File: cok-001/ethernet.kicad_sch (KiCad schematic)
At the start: 1 part, among them J3501 RJ45_Amphenol_RJMG1BD3B8K1ANR

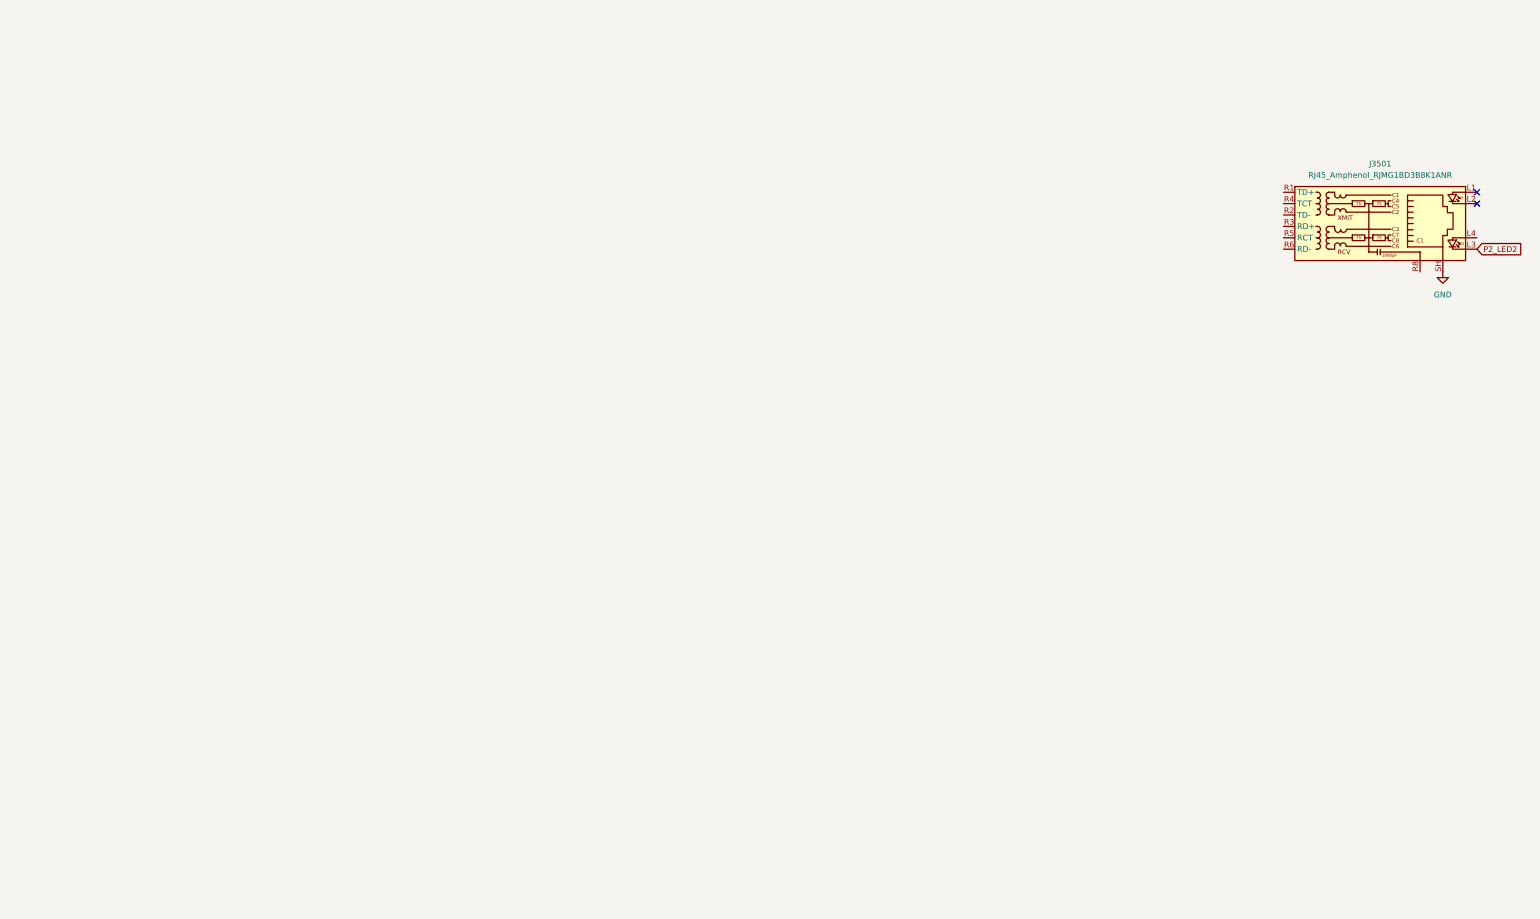
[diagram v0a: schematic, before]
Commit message: ethernet
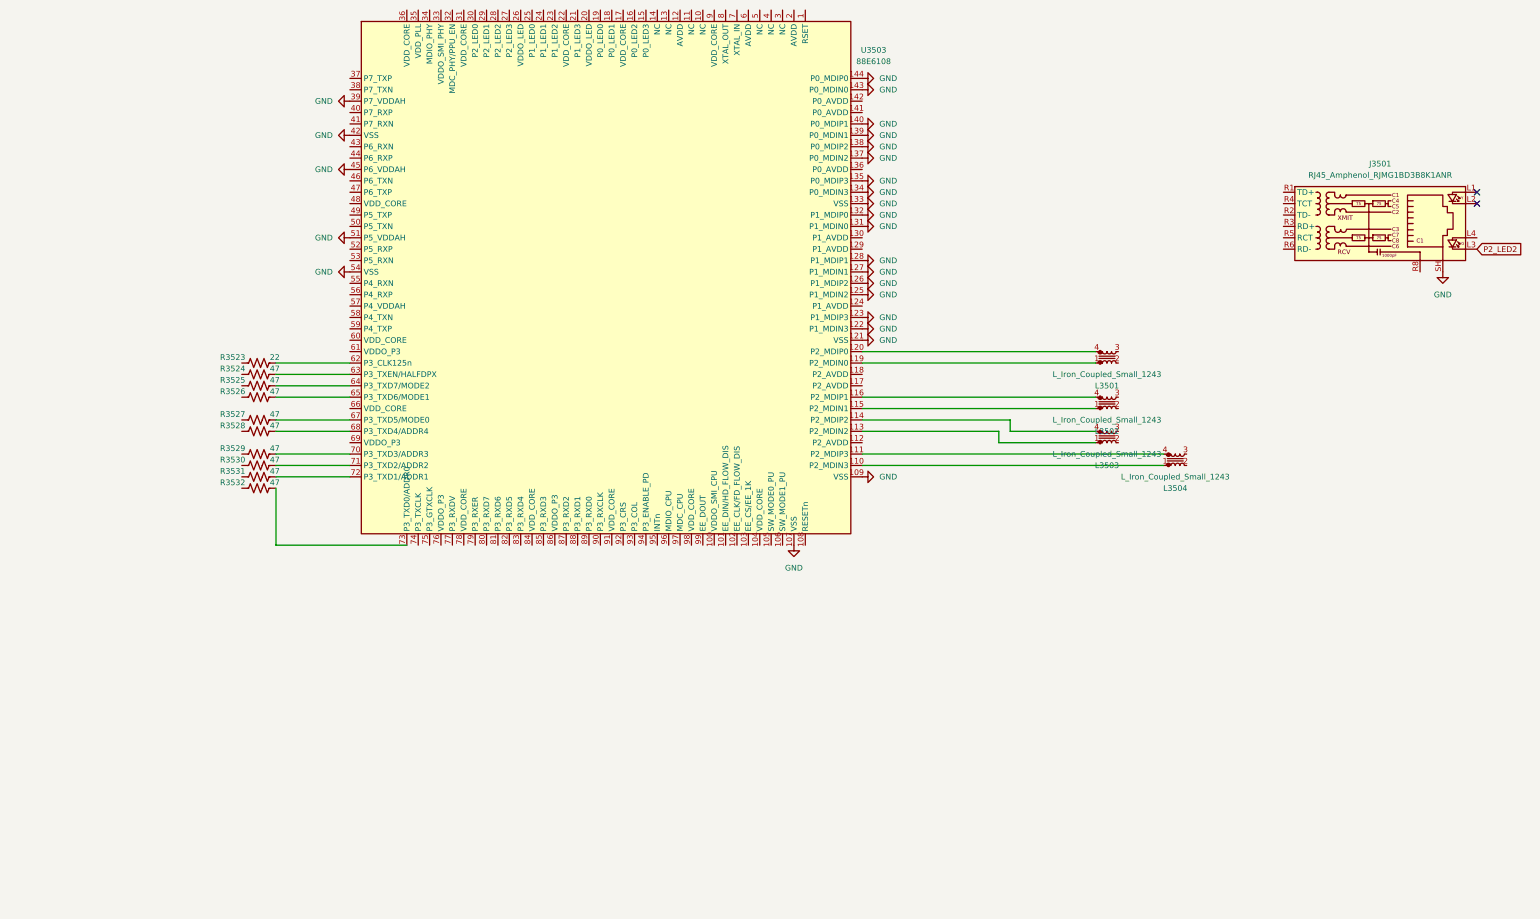
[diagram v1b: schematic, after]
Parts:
- added L3501, L3502, L3503, L3504: L_Iron_Coupled_Small_1243, Inductor_SMD:L_CommonModeChoke_Coilcraft_0805USB, symbol Device:L_Iron_Coupled_Small_1243
- added R3523: 22, Resistor_SMD:R_0402_1005Metric, symbol Device:R_US
- added R3524, R3525, R3526, R3527, R3528, R3529, R3530, R3531, R3532: 47, Resistor_SMD:R_0402_1005Metric, symbol Device:R_US
- added U3503: 88E6108, Package_QFP:LQFP-144_20x20mm_P0.5mm, symbol PS3:88E6108
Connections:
- net GND: now also U3503.107 (VSS), U3503.109 (VSS), U3503.121 (VSS), U3503.122 (P1_MDIN3), U3503.123 (P1_MDIP3), U3503.125 (P1_MDIN2), U3503.126 (P1_MDIP2), U3503.127 (P1_MDIN1), U3503.128 (P1_MDIP1), U3503.131 (P1_MDIN0), U3503.132 (P1_MDIP0), U3503.133 (VSS), U3503.134 (P0_MDIN3), U3503.135 (P0_MDIP3), U3503.137 (P0_MDIN2), U3503.138 (P0_MDIP2), U3503.139 (P0_MDIN1), U3503.140 (P0_MDIP1), U3503.143 (P0_MDIN0), U3503.144 (P0_MDIP0), U3503.39 (P7_VDDAH), U3503.42 (VSS), U3503.45 (P6_VDDAH), U3503.51 (P5_VDDAH), U3503.54 (VSS)
- new net: R3526.2, U3503.65 (P3_TXD6/MODE1)
- new net: R3524.2, U3503.63 (P3_TXEN/HALFDPX)
- new net: L3502.1, U3503.115 (P2_MDIN1)
- new net: L3502.4, U3503.116 (P2_MDIP1)
- new net: R3525.2, U3503.64 (P3_TXD7/MODE2)
- new net: L3501.1, U3503.119 (P2_MDIN0)
- new net: L3501.4, U3503.120 (P2_MDIP0)
- new net: L3503.1, U3503.113 (P2_MDIN2)
- new net: L3503.4, U3503.114 (P2_MDIP2)
- new net: R3523.2, U3503.62 (P3_CLK125n)
- new net: R3527.2, U3503.67 (P3_TXD5/MODE0)
- new net: R3529.2, U3503.70 (P3_TXD3/ADDR3)
- new net: L3504.1, U3503.110 (P2_MDIN3)
- new net: L3504.4, U3503.111 (P2_MDIP3)
- new net: R3530.2, U3503.71 (P3_TXD2/ADDR2)
- new net: R3528.2, U3503.68 (P3_TXD4/ADDR4)
- new net: R3532.2, U3503.73 (P3_TXD0/ADDR0)
- new net: R3531.2, U3503.72 (P3_TXD1/ADDR1)

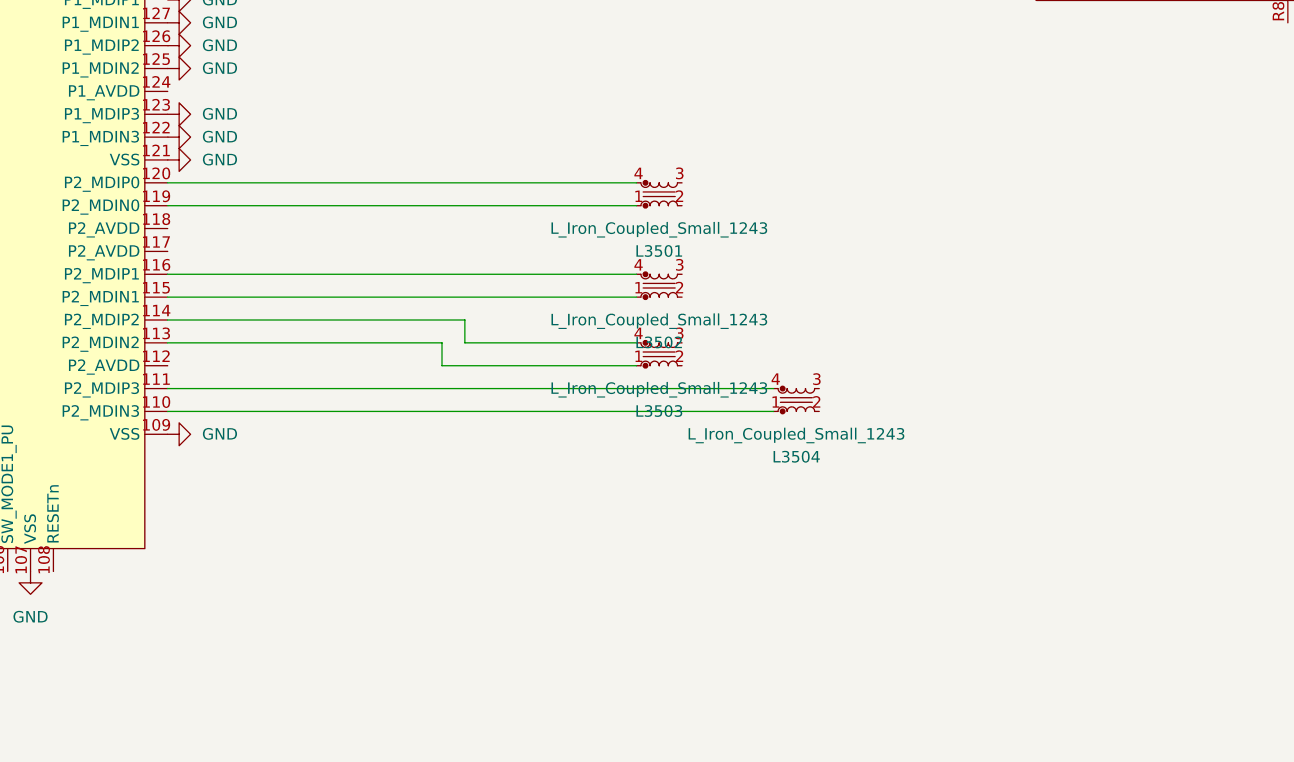
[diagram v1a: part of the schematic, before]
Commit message: av
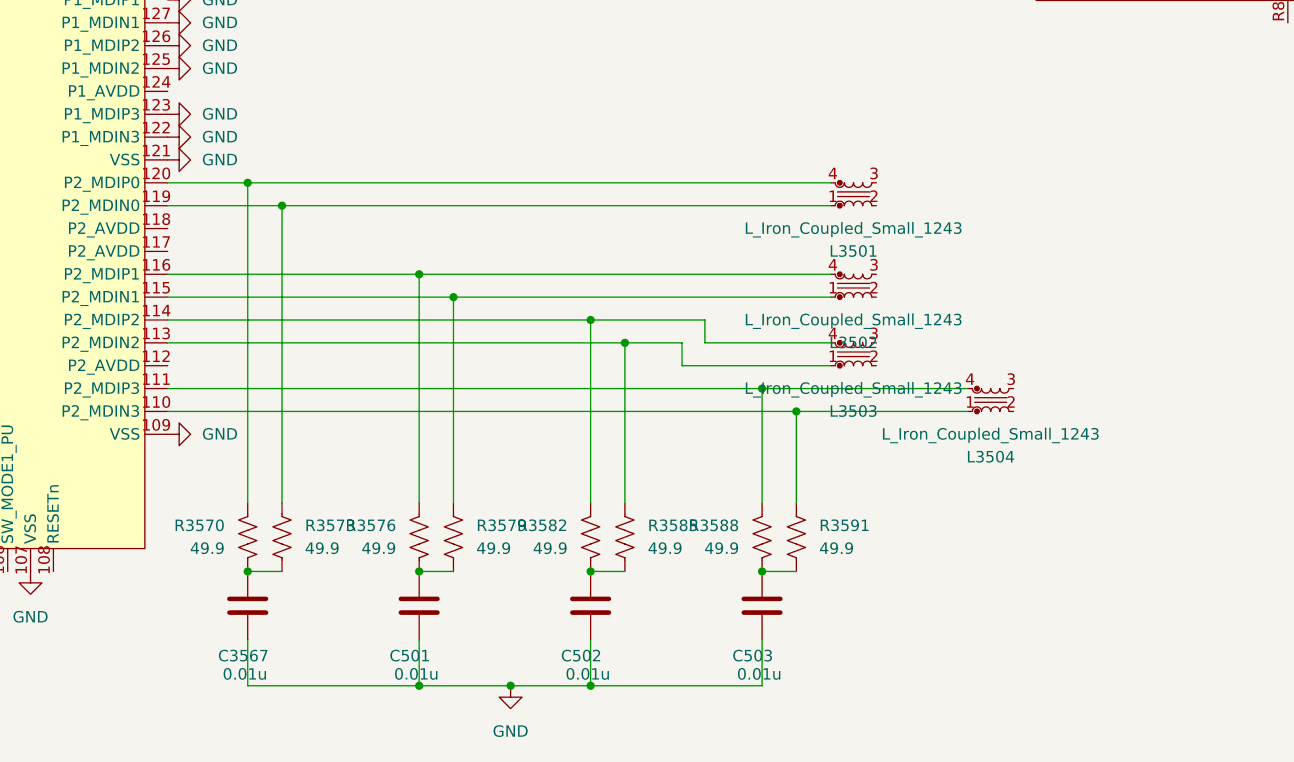
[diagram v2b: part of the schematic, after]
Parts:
- added C3567, C501, C502, C503: 0.01u, Capacitor_SMD:C_0402_1005Metric, symbol Device:C
- added R3570, R3573, R3576, R3579, R3582, R3585, R3588, R3591: 49.9, Resistor_SMD:R_0402_1005Metric, symbol Device:R_US
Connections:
- net GND: now also C3567.2, C501.2, C502.2, C503.2
- net at L3502.1, U3503.115 (P2_MDIN1): now also R3579.2
- net at L3502.4, U3503.116 (P2_MDIP1): now also R3576.2
- net at L3501.1, U3503.119 (P2_MDIN0): now also R3573.2
- net at L3501.4, U3503.120 (P2_MDIP0): now also R3570.2
- net at L3503.1, U3503.113 (P2_MDIN2): now also R3585.2
- net at L3503.4, U3503.114 (P2_MDIP2): now also R3582.2
- net at L3504.1, U3503.110 (P2_MDIN3): now also R3591.2
- net at L3504.4, U3503.111 (P2_MDIP3): now also R3588.2
- new net: C502.1, R3582.1, R3585.1
- new net: C3567.1, R3570.1, R3573.1
- new net: C503.1, R3588.1, R3591.1
- new net: C501.1, R3576.1, R3579.1
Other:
- moved on the sheet: L3501, L3502, L3503, L3504

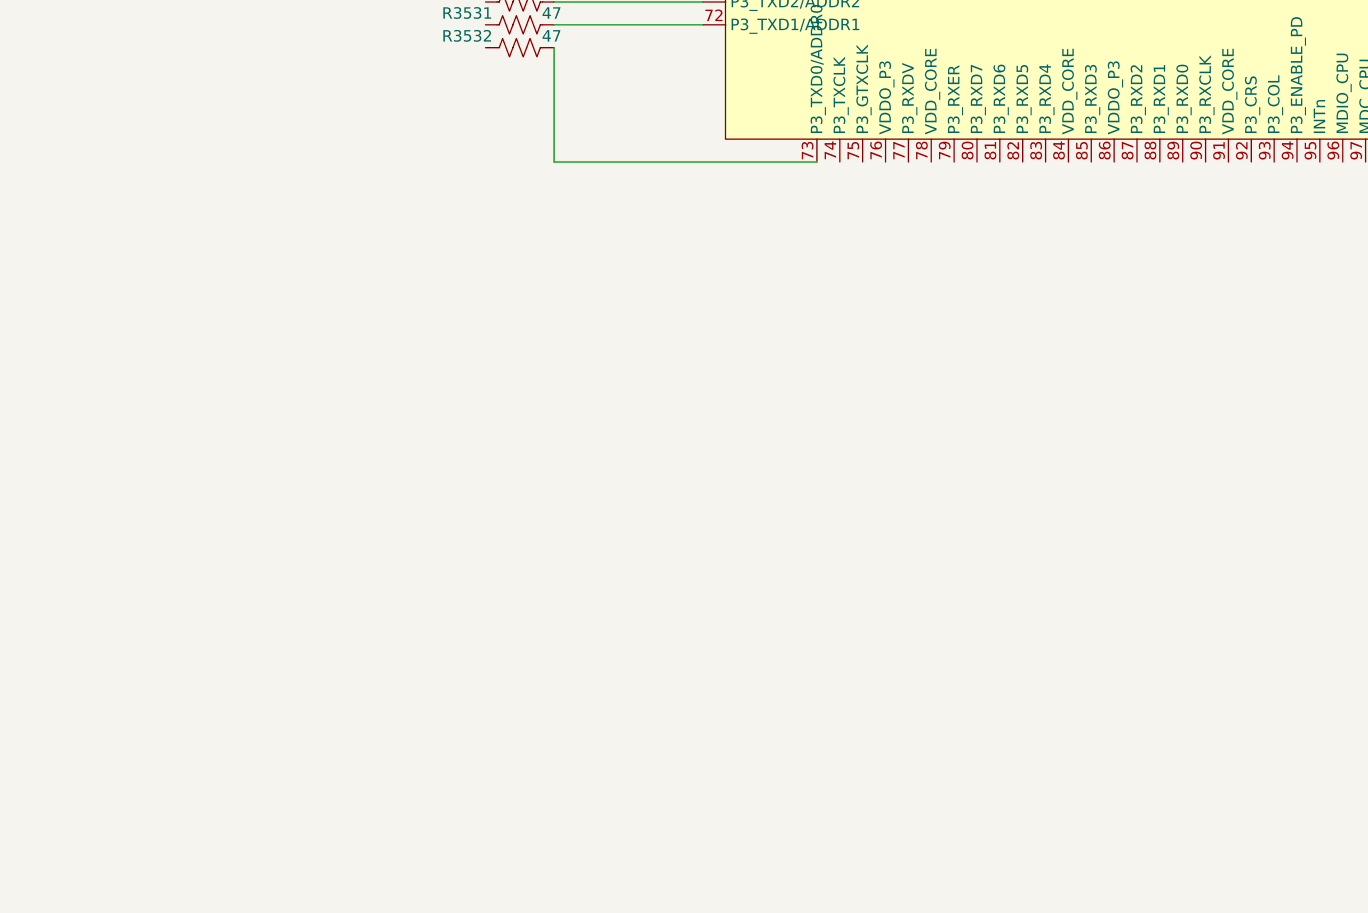
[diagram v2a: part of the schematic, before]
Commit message: aj
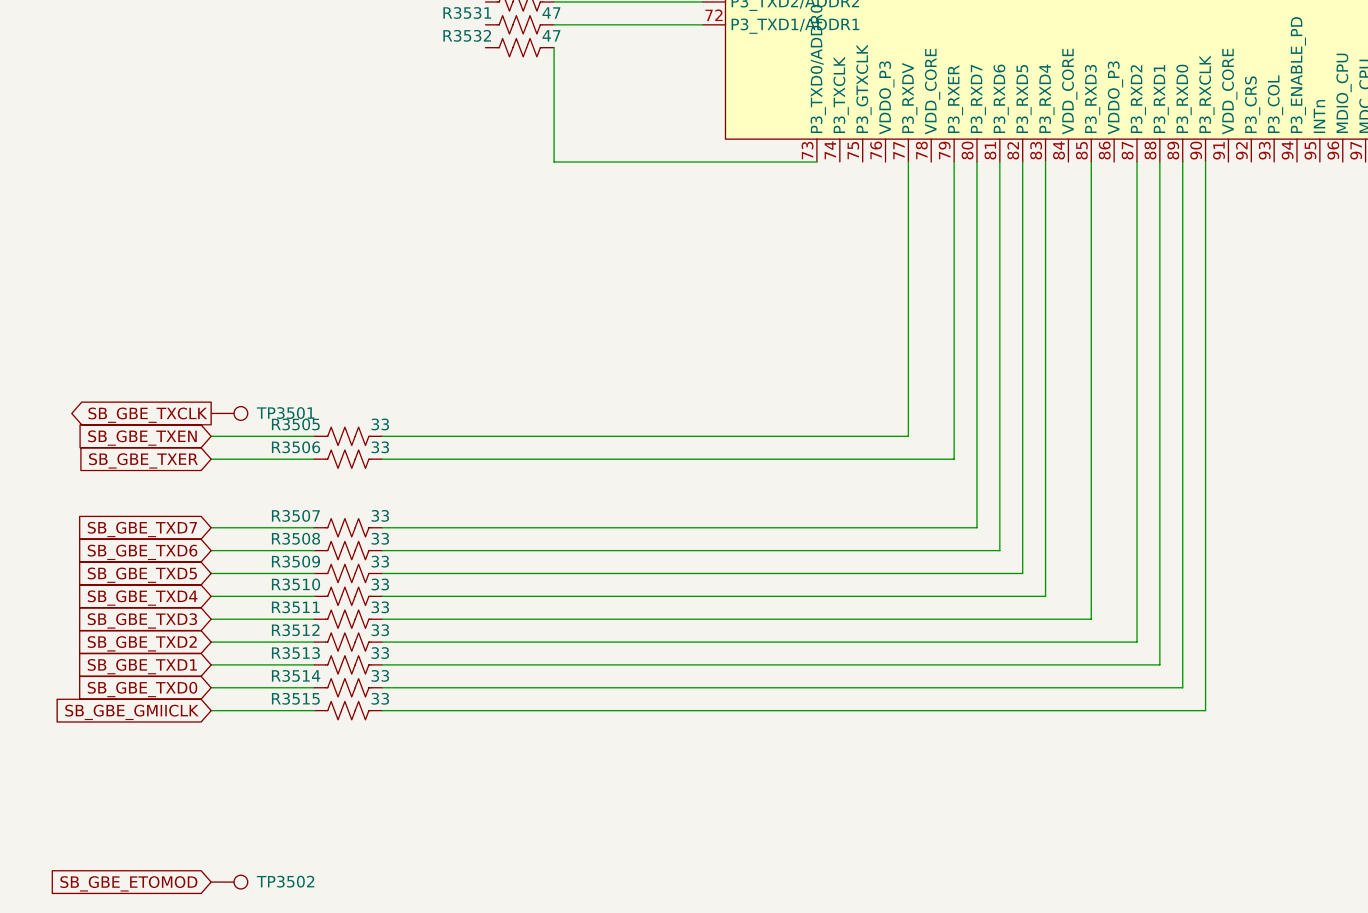
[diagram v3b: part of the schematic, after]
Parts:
- added R3505, R3506, R3507, R3508, R3509, R3510, R3511, R3512, R3513, R3514, R3515: 33, Resistor_SMD:R_0402_1005Metric, symbol Device:R_US
- added TP3501, TP3502: TestPoint, TestPoint:TestPoint_Pad_1.0x1.0mm, symbol Connector:TestPoint
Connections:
- net at U3503.77 (P3_RXDV): now also R3505.2
- net at U3503.79 (P3_RXER): now also R3506.2
- net at U3503.80 (P3_RXD7): now also R3507.2
- net at U3503.81 (P3_RXD6): now also R3508.2
- net at U3503.82 (P3_RXD5): now also R3509.2
- net at U3503.83 (P3_RXD4): now also R3510.2
- net at U3503.85 (P3_RXD3): now also R3511.2
- net at U3503.87 (P3_RXD2): now also R3512.2
- net at U3503.88 (P3_RXD1): now also R3513.2
- net at U3503.89 (P3_RXD0): now also R3514.2
- net at U3503.90 (P3_RXCLK): now also R3515.2
- new net SB_GBE_ETOMOD: TP3502.1
- new net SB_GBE_GMIICLK: R3515.1
- new net SB_GBE_TXCLK: TP3501.1
- new net SB_GBE_TXD0: R3514.1
- new net SB_GBE_TXD1: R3513.1
- new net SB_GBE_TXD2: R3512.1
- new net SB_GBE_TXD3: R3511.1
- new net SB_GBE_TXD4: R3510.1
- new net SB_GBE_TXD5: R3509.1
- new net SB_GBE_TXD6: R3508.1
- new net SB_GBE_TXD7: R3507.1
- new net SB_GBE_TXEN: R3505.1
- new net SB_GBE_TXER: R3506.1

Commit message: update to 9
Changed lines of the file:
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@@
 (kicad_sch
-	(version 20231120)
+	(version 20250114)
 	(generator "eeschema")
-	(generator_version "8.0")
+	(generator_version "9.0")
 	(paper "A4")
 	(junction
